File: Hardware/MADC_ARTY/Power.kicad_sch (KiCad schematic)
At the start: 53 parts, among them U17 TSR3-2450N, U26 ADP7182ACPZN, U27 ADP7182ACPZN, U28 ADP7142ACPZN, U5 ADP7142ARDZ-3.3, U6 ADP5070AREZ

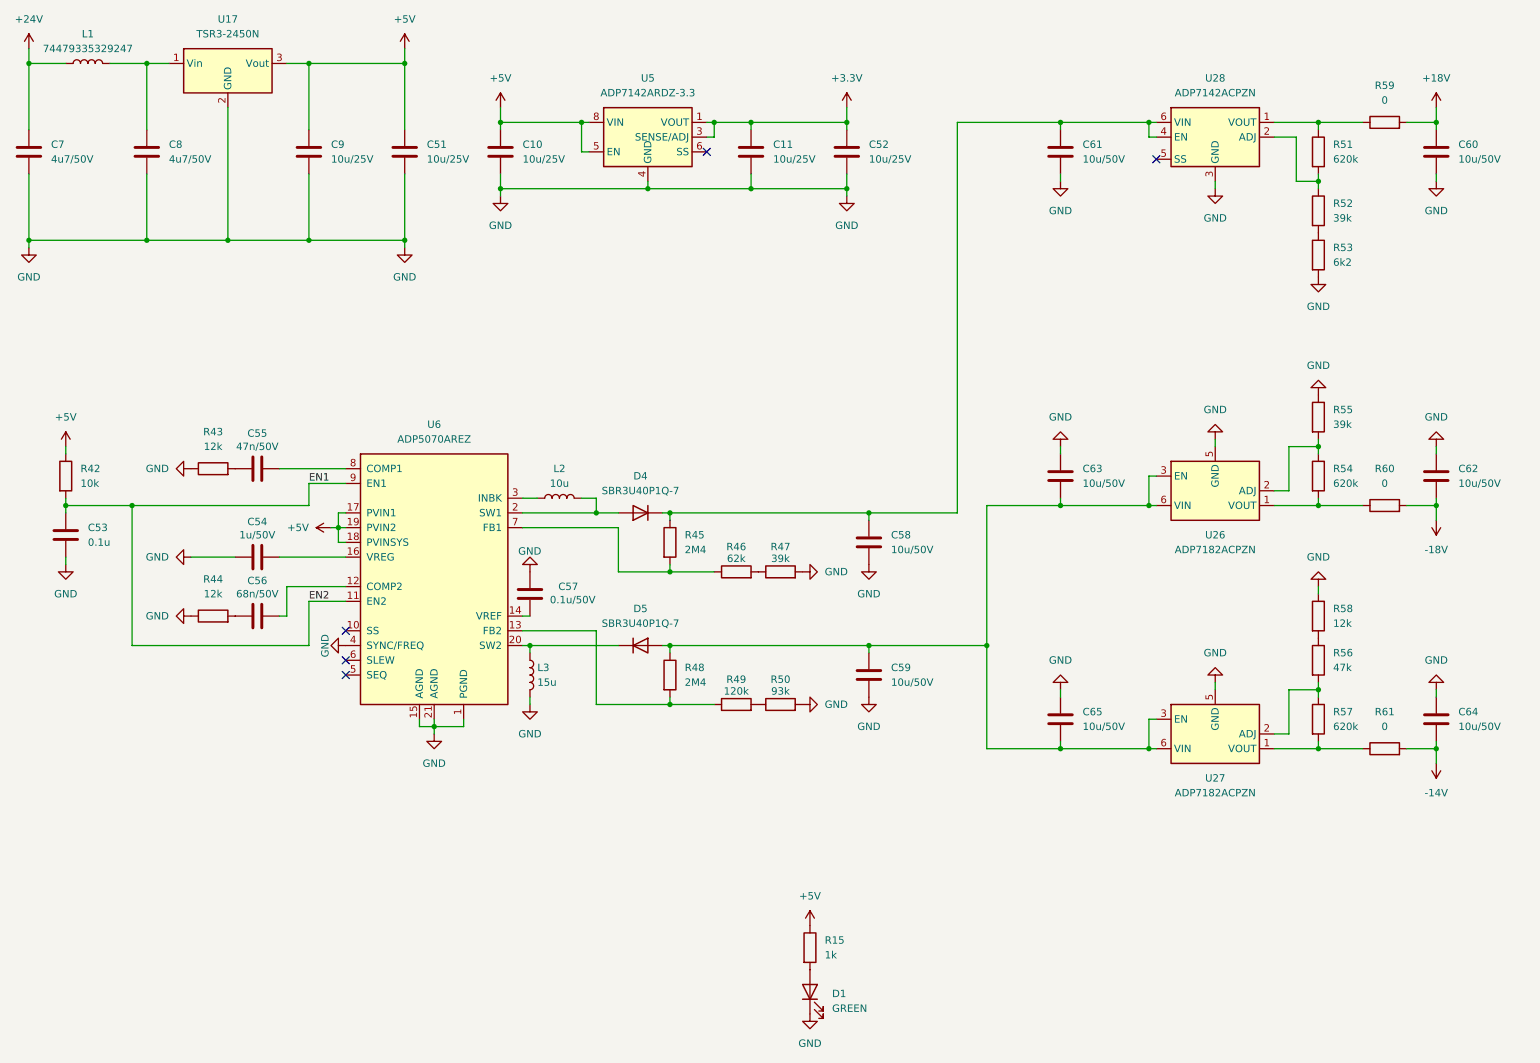
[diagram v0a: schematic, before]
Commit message: Schematic
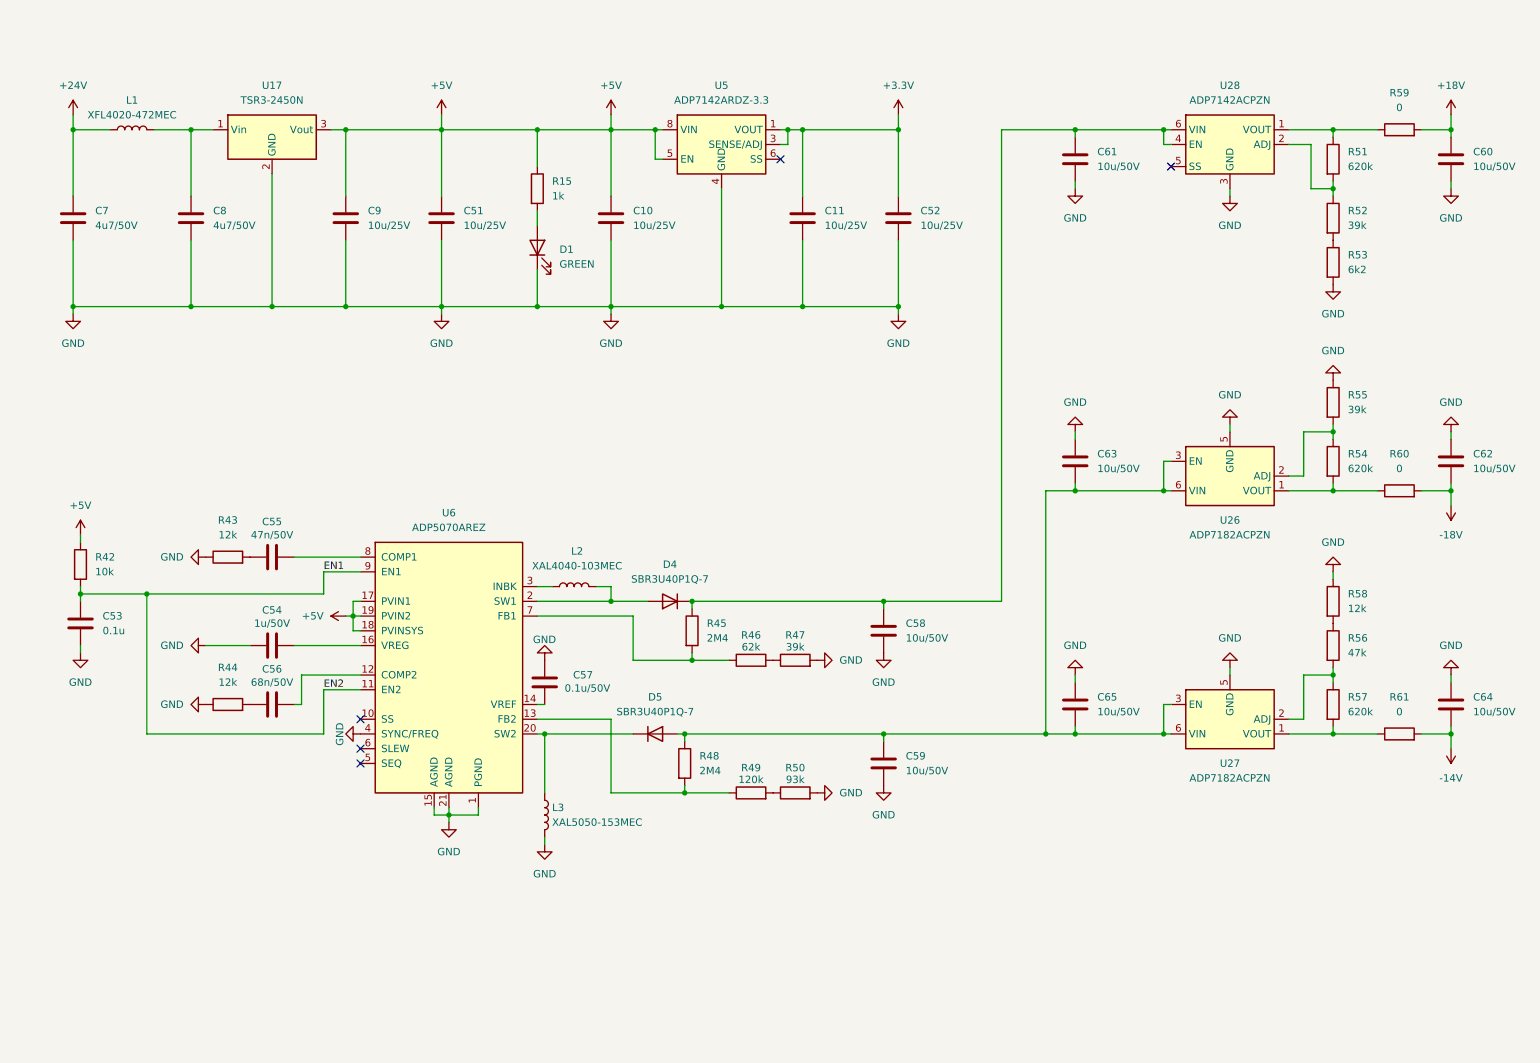
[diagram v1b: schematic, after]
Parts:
- L1: value 74479335329247 -> XFL4020-472MEC; footprint (none) -> Inductor_SMD:L_Coilcraft_XAL4020-XXX
- L2: value 10u -> XAL4040-103MEC; footprint (none) -> Inductor_SMD:L_Coilcraft_XAL4040-XXX
- L3: value 15u -> XAL5050-153MEC; footprint (none) -> Inductor_SMD:L_Coilcraft_XAL5050-XXX
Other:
- moved on the sheet: C10, C11, C51, C52, C53, C54, C55, C56, C57, C58, C59, C60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
